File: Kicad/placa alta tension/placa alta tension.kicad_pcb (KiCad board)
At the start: 2 copper layers, 94 x 80 mm, 53 parts, among them J1 Screw_Terminal_01x02, J2 Screw_Terminal_01x02, J3 Screw_Terminal_01x02, J4 Conn_01x05_Socket, Q1 2N7000, Q2 2N7000, U1 MOC3023M, U2 4N25, U3 74HC14, U4 MOC3023M

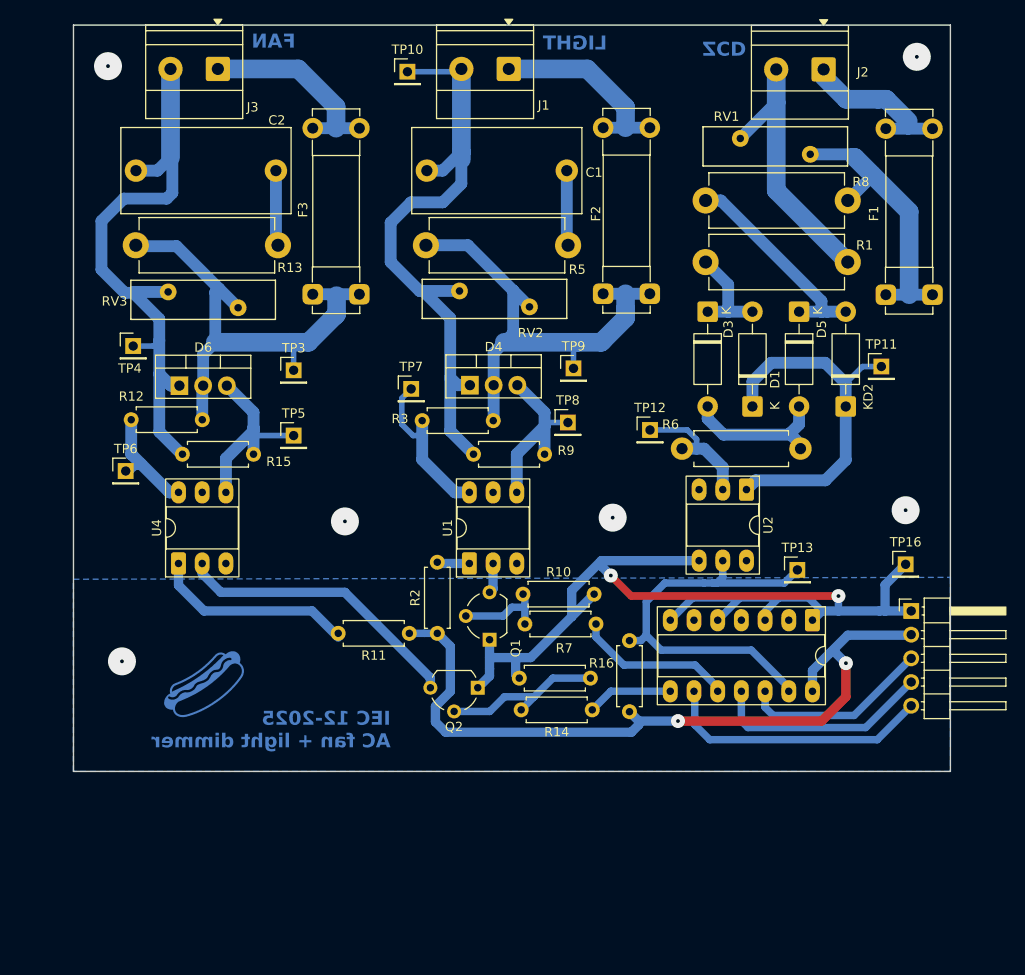
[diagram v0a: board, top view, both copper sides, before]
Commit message: avances placa
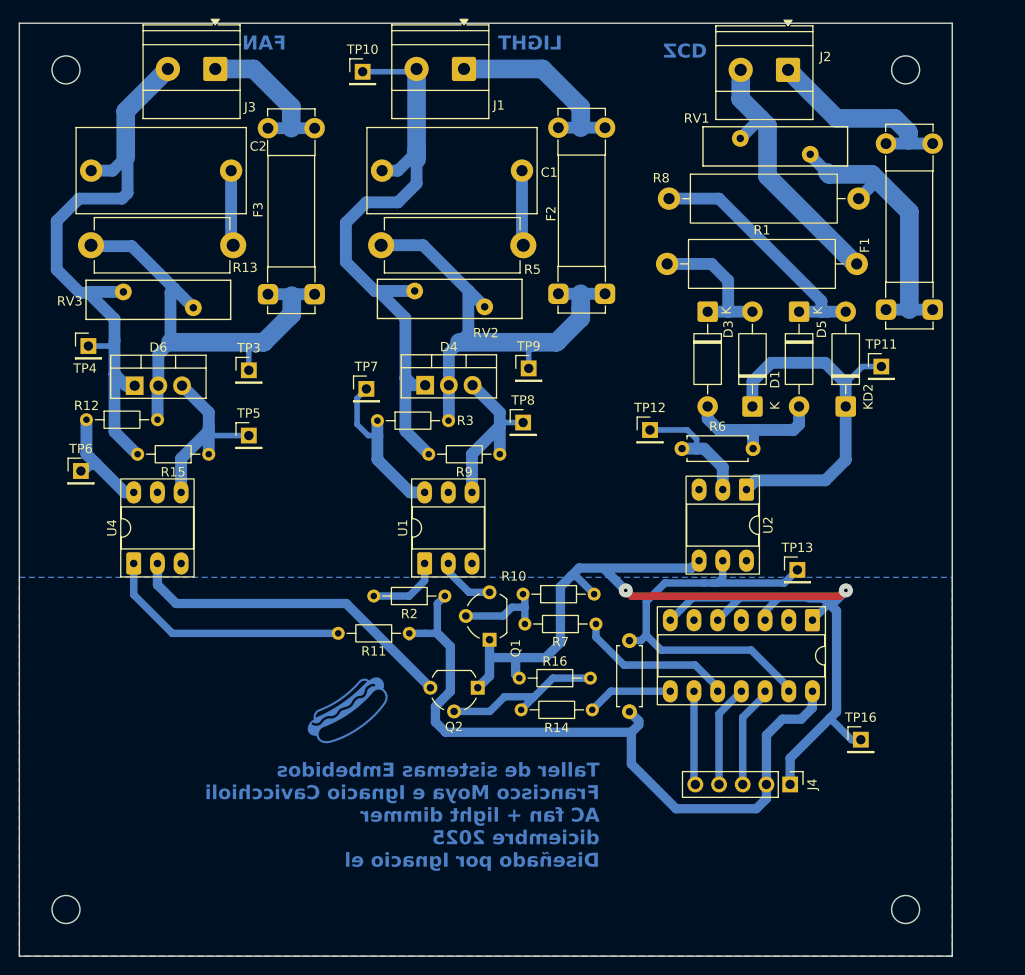
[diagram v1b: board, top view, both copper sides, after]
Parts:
- D4, D6: value Generic_Triac_A1A2G -> BTA06-600C
- J4: footprint Connector_PinHeader_2.54mm:PinHeader_1x05_P2.54mm_Horizontal -> Connector_PinHeader_2.54mm:PinHeader_1x05_P2.54mm_Vertical
- R1, R8: footprint Resistor_THT:R_Axial_DIN0614_L14.3mm_D5.7mm_P15.24mm_Horizontal -> Resistor_THT:R_Axial_DIN0516_L15.5mm_D5.0mm_P20.32mm_Horizontal
- R10, R11, R12, R14, R15, R16, R2, R3, R7, R9: footprint Resistor_THT:R_Axial_DIN0207_L6.3mm_D2.5mm_P7.62mm_Horizontal -> Resistor_THT:R_Axial_DIN0204_L3.6mm_D1.6mm_P7.62mm_Horizontal
- R13, R5: value 2.4k -> 1k
- R6: footprint Resistor_THT:R_Axial_DIN0411_L9.9mm_D3.6mm_P12.70mm_Horizontal -> Resistor_THT:R_Axial_DIN0207_L6.3mm_D2.5mm_P7.62mm_Horizontal
- moved J4 22.7 mm to (191.4, 133.2), turned to -90 degrees
- moved TP16 19.4 mm to (199.0, 128.4)
- moved G*** 15.7 mm to (144.2, 125.4)
- moved C2 4.80 mm to (131.5, 67.4)
- moved F3 4.80 mm to (135.4, 80.7)
- moved R12 4.80 mm to (116.0, 94.1)
- moved R13 4.80 mm to (131.7, 75.4)
- moved R15 4.80 mm to (129.1, 97.8)
- moved R5 4.80 mm to (162.8, 75.4)
- moved TP10 4.80 mm to (145.6, 56.8)
- moved TP7 4.80 mm to (146.0, 90.8)
- moved D6 4.80 mm to (121.2, 90.5)
- moved RV3 4.80 mm to (127.5, 82.1)
- moved TP4 4.80 mm to (116.2, 86.2)
- moved TP6 4.80 mm to (115.4, 99.6)
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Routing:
- net /FAN: track 29.0 -> 10.2 mm
- net GND: track 109.8 -> 124.6 mm
- net /LIGHT: track 23.7 -> 11.0 mm
- net /ZCD: track 20.3 -> 11.0 mm
- net Net-(R11-Pad2): track 21.8 -> 27.0 mm
- net Net-(Q2-D): track 31.2 -> 36.1 mm
- net DIMMING_LINE: track 21.6 -> 17.1 mm
- net Net-(R2-Pad2): track 3.49 -> 7.98 mm
- net Net-(D1-A): track 10.3 -> 14.6 mm
- net Net-(J2-Pin_1): track 17.6 -> 21.9 mm
- net +5V: track 82.0 -> 77.9 mm, vias 2 -> 0
- net /HV9: track 21.8 -> 25.8 mm
- net Net-(Q1-D): track 3.25 -> 6.21 mm
- net Net-(D6-A1): track 65.4 -> 67.2 mm
- net N: track 30.9 -> 31.9 mm
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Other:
- board size 94 x 80 mm -> 100 x 100 mm
- board text added: "Taller de sistemas Embebidos Francisco Moya e Ignacio Cavicchioli AC fan + light dimmer diciembre 2025 Diseñado por Ignacio el"
- board text removed: "IEC 12-2025 AC fan + light dimmer"
